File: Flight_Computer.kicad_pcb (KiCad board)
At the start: 4 copper layers, 100 x 66.2 mm, 67 parts, among them J1 PYRO, J2 PYRO, J3 Conn_01x04, J5 Conn_01x02_Pin, J6 Conn_01x09_Socket, J9 Conn_01x02_Pin, Q1 IRLZ44N, Q2 IRLZ44N, SW2 SW_Push, SW3 SW_Push, U1 TLV1117-33, U2 ESP32-S3-WROOM-1, U6 LPS22HH, U7 MAX-M8C, U8 LSM6DS3, U9 W25Q16JVSS

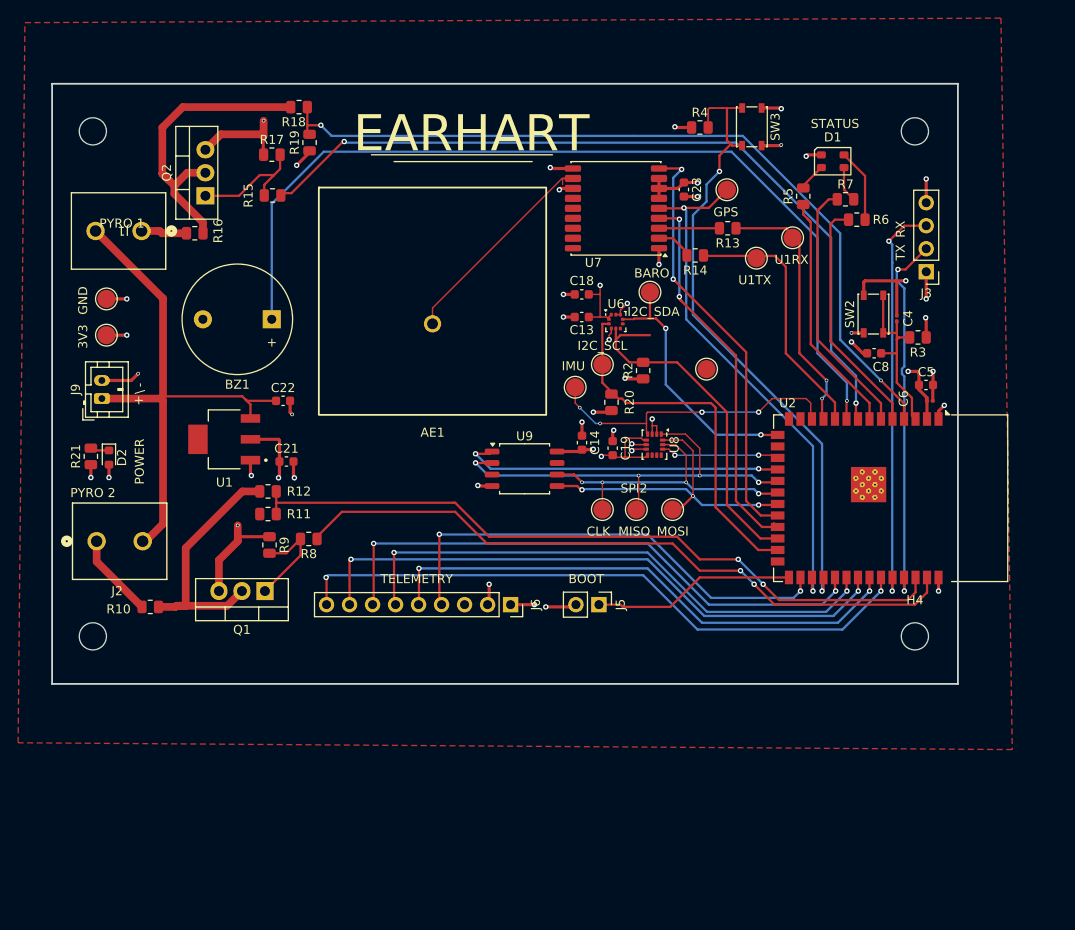
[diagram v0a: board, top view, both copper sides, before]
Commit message: Upload final pcb and schematic version
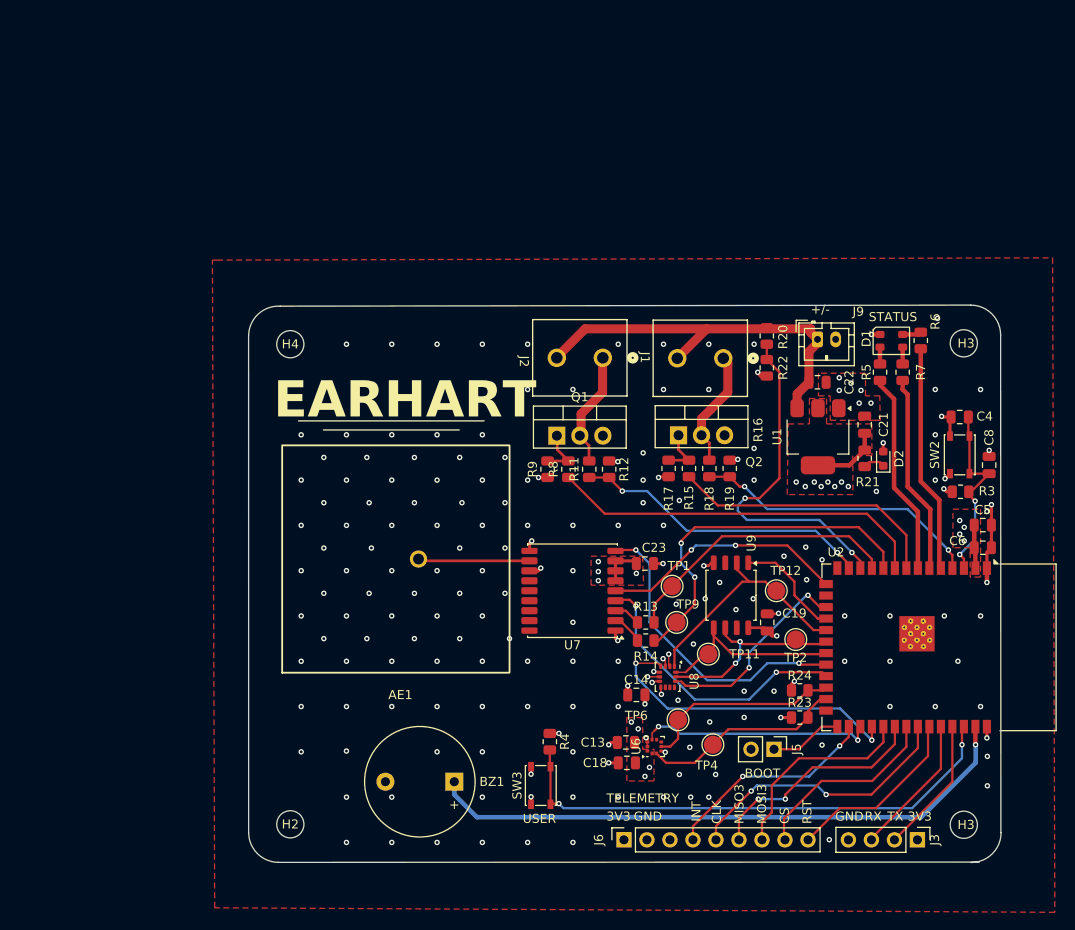
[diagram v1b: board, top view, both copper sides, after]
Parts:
- removed H1: MountingHole, MountingHole:MountingHole_3mm
- removed the H3 at (212.8, 46.5)
- removed R10, R16: 1, Resistor_SMD:R_0805_2012Metric
- removed R2: 4.7K, Resistor_SMD:R_0805_2012Metric
- removed TP10, TP13, TP15, TP16, TP7: TestPoint, TestPoint:TestPoint_Pad_D2.0mm
- added H3: MountingHole, MountingHole:MountingHole_3mm, F.Cu at (218.2, 123.0)
- added H3: MountingHole, MountingHole:MountingHole_3mm, F.Cu at (218.2, 69.9)
- added R22: 10K, Resistor_SMD:R_0805_2012Metric, F.Cu at (196.4, 72.6)
- added R23: 4.7K, Resistor_SMD:R_0805_2012Metric, F.Cu at (200.0, 111.2)
- added R24: 4.7K, Resistor_SMD:R_0805_2012Metric, F.Cu at (200.0, 108.2)
- C13, C14, C18, C19, C21, C22, C23, C5, C8: footprint Capacitor_SMD:C_0603_1608Metric -> Capacitor_SMD:C_0805_2012Metric
- C4, C6: footprint Capacitor_SMD:C_0201_0603Metric -> Capacitor_SMD:C_0805_2012Metric
- R20: value 4.7K -> 10K
- U1: footprint TLV1117-33CDCY:SOT230P700X180-4N -> Package_TO_SOT_SMD:SOT-223-3_TabPin2
- moved D2 85.5 mm to (209.3, 82.6), turned to 90 degrees
- moved R21 85.4 mm to (207.2, 82.6), turned to -90 degrees
- moved J9 79.3 mm to (202.0, 69.5), turned to 0 degrees
- moved SW3 76.4 mm to (171.5, 118.7), turned to 90 degrees
- moved H4 76.1 mm to (143.8, 70.0)
- moved R4 69.8 mm to (172.5, 113.9), turned to -90 degrees
- moved J1 65.7 mm to (191.6, 71.6)
- moved U1 65.6 mm to (202.1, 80.2), turned to -90 degrees
- moved C21 64.0 mm to (207.2, 78.9), turned to 90 degrees
- moved J3 62.7 mm to (213.0, 124.7), turned to -90 degrees
- moved R18 60.4 mm to (190.1, 83.7), turned to 90 degrees
- moved J2 59.4 mm to (178.3, 71.5), turned to 180 degrees
- moved C22 59.0 mm to (202.0, 74.2)
- moved R19 58.7 mm to (192.3, 83.7), turned to -90 degrees
- moved Q2 58.5 mm to (186.7, 80.1), turned to 0 degrees
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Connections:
- Q1 pad 2: Net-(Q1-D) -> Net-(J2-Pin_1)
- Q2 pad 2: Net-(Q2-D) -> Net-(J1-Pin_1)
- R11 pad 2: Net-(Q1-D) -> Net-(J2-Pin_1)
- R18 pad 2: Net-(Q2-D) -> Net-(J1-Pin_1)
- R20 pad 1: +3.3V -> /BATT_IN
- R20 pad 2: I2C_SCL -> /BATT_SENSE
- U2 pad 12: IMU_INT -> /BATT_SENSE
- U2 pad 13: unconnected-(U2-USB_D--Pad13) -> /SENSE_1
- U2 pad 15: BARO_INT -> GPS_EXTINT
- U2 pad 29: GPS_EXTINT -> BARO_INT
- U2 pad 30: /BUTT_0 -> IMU_INT
- U2 pad 38: /SENSE_1 -> /BUTT_0
- U2 pad 39: /PYRO_1 -> /BUZZER
- U2 pad 9: /BUZZER -> /PYRO_1
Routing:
- net /PYRO_2: track 88.8 -> 30.3 mm, vias 2 -> 0
- net /SENSE_2: track 90.3 -> 31.9 mm
- net GND: track 95.0 -> 39.8 mm, vias 34 -> 184
- net /TELE_RST: track 70.1 -> 20.4 mm, vias 2 -> 0
- net /SENSE_1: track 79.5 -> 33.1 mm
- net /TELE_CS: track 66.3 -> 21.4 mm, vias 2 -> 0
- net /MOSI3: track 63.0 -> 22.5 mm, vias 2 -> 0
- net /BATT_SENSE: track 0.00 -> 38.4 mm, vias 0 -> 2
- net /MISO3: track 61.3 -> 25.2 mm
- net /BUZZER: track 100.7 -> 66.5 mm
- net Net-(Q2-D): track 33.7 -> 0.00 mm
- net /PYRO_1: track 74.9 -> 41.9 mm, vias 2 -> 0
- net +3.3V: track 61.6 -> 28.8 mm, vias 15 -> 29
- net GPS_EXTINT: track 58.1 -> 27.1 mm
- net /MCU_RX: track 45.1 -> 15.4 mm, vias 2 -> 0
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- added copper zone on F.Cu, net +3.3V
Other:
- board size 100 x 66.2 mm -> 83.1 x 61.5 mm
- board text added: "+/-"
- board text added: "CS"
- board text added: "INT"
- board text added: "MISO3"
- board text added: "MOSI3"
- board text added: "R16"
- board text added: "RST"
- board text added: "USER"
- board text removed: "+"
- board text removed: "-"
- board text removed: "BARO"
- board text removed: "GPS"
- board text removed: "I2C_SCL"
- board text removed: "I2C_SDA"
- board text removed: "IMU"
- board text removed: "MISO"
- board text removed: "MOSI"
- board text removed: "POWER"
- board text removed: "PYRO 1"
- board text removed: "PYRO 2"
- board text removed: "SPI2"
- board text removed: "U1RX"
- board text removed: "U1TX"
- board text removed: "\"
